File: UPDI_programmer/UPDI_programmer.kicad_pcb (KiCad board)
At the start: 2 copper layers, 74.3 x 25.4 mm, 30 parts, among them J1 UPDI, J2 ICSP, J3 USB_A, U1 ATmega168P-20AU, U2 FT230XS, Y1 16MHz

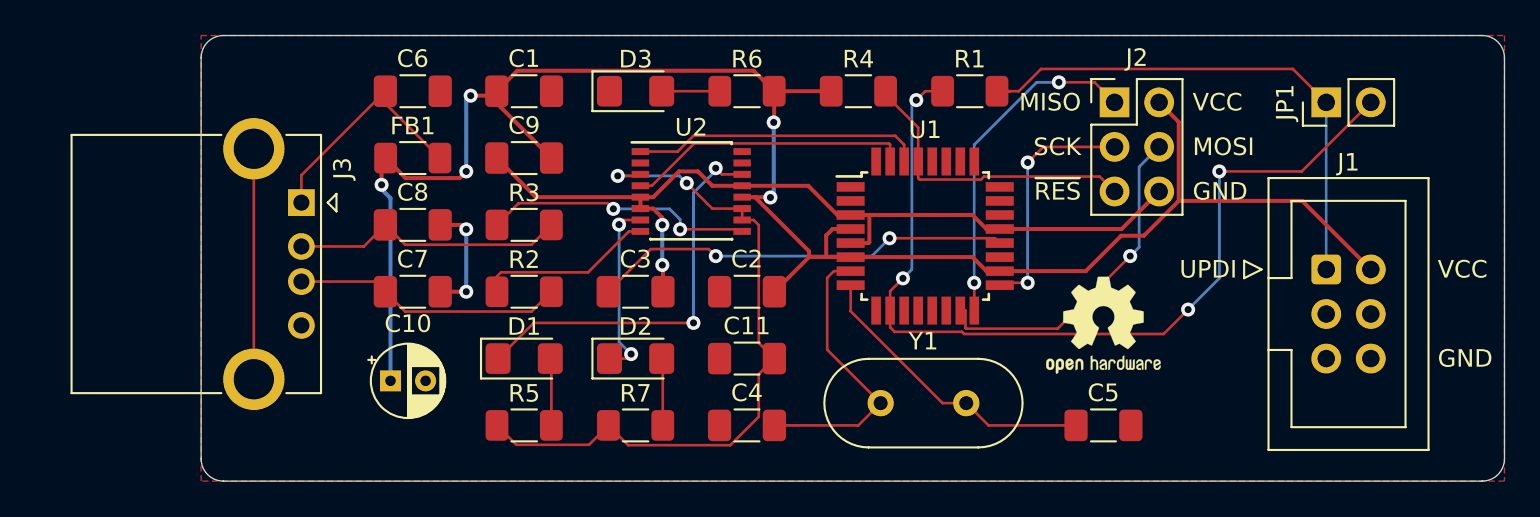
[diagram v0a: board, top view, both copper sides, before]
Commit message: UPDI PCB RC1
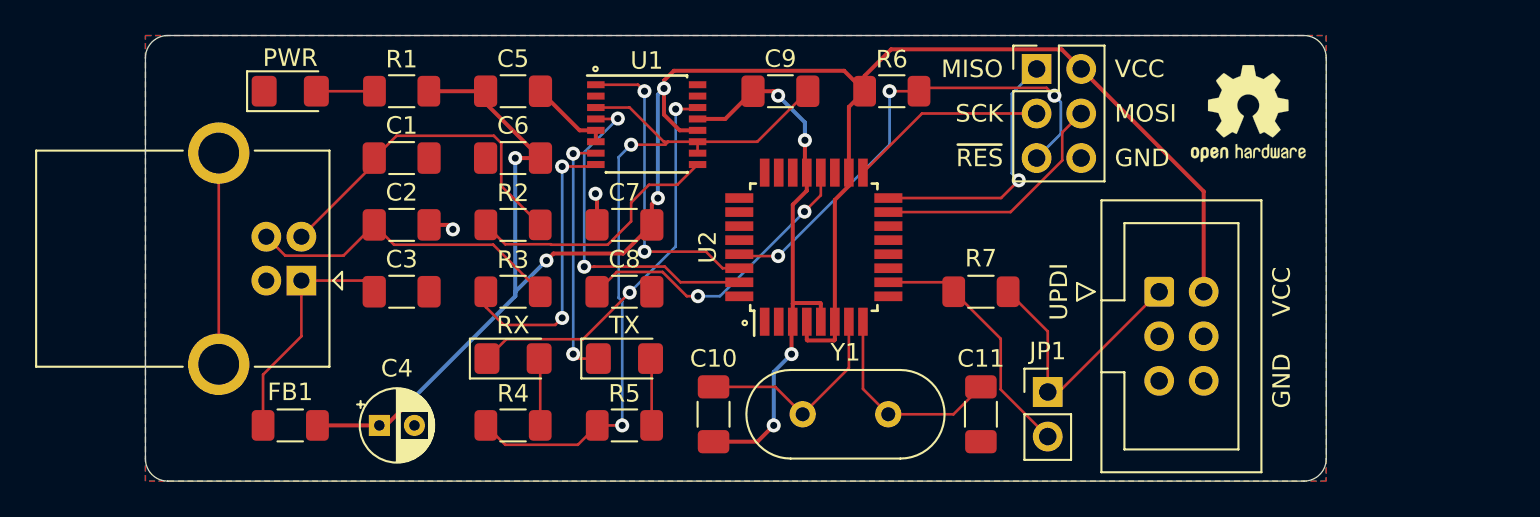
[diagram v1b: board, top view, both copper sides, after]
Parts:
- added QR*****: https://tinyurl.com/ghdbks, QR:kicad-simple, B.Cu at (160.0, 61.6)
- added REF**: KiCad-Logo2_5mm_SilkScreen, Symbol:KiCad-Logo2_5mm_SilkScreen, B.Cu at (128.9, 66.0)
- J3: value USB_A -> USB_B; footprint Connector_USB:USB_A_CONNFLY_DS1095-WNR0 -> Connector_USB:USB_B_OST_USB-B1HSxx_Horizontal
- moved JP1 22.9 mm to (150.5, 75.6), turned to 0 degrees
- moved D3 19.7 mm to (107.3, 58.4)
- moved R1 19.7 mm to (113.7, 58.4)
- moved FB1 16.8 mm to (107.3, 77.5), turned to 180 degrees
- moved C9 15.4 mm to (135.3, 58.4)
- moved REF** 14.6 mm to (161.9, 59.7)
- moved C3 11.4 mm to (113.7, 69.8)
- moved R7 11.4 mm to (146.7, 69.8)
- moved J1 9.61 mm to (156.8, 69.8)
- moved C7 7.96 mm to (126.4, 66.0)
- moved C11 7.01 mm to (146.7, 76.8), turned to 270 degrees
- moved U2 6.38 mm to (137.2, 67.3), turned to 90 degrees
- moved J2 4.84 mm to (149.9, 57.1)
- moved U1 4.58 mm to (127.6, 60.3)
- moved Y1 4.49 mm to (136.5, 76.8)
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- renumbered C8 to C1, C4 to C10, C5 to C11, C7 to C2, C6 to C3, C10 to C4, C1 to C5, C9 to C6, C2 to C7, C3 to C8, C11 to C9, R6 to R1, R3 to R2, R2 to R3, R5 to R4, R7 to R5, R4 to R6, R1 to R7, U2 to U1, U1 to U2
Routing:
- net UPDI: track 51.9 -> 14.4 mm, vias 4 -> 0
- net GND: track 58.2 -> 40.1 mm, vias 4 -> 6
- net Net-(J1-Pad1): track 30.3 -> 15.4 mm
- net ~RESET: track 17.4 -> 28.2 mm, vias 0 -> 3
- net Net-(C8-Pad1): track 24.0 -> 17.5 mm
- net USBD+: track 10.1 -> 16.4 mm, vias 0 -> 2
- net Net-(C11-Pad1): track 17.0 -> 11.8 mm
- net MOSI: track 19.3 -> 14.3 mm, vias 1 -> 0
- net MISO: track 19.4 -> 15.0 mm, vias 2 -> 1
- net Net-(C10-Pad2): track 16.5 -> 12.1 mm
- net VCC: track 109.1 -> 113.5 mm
- net Net-(C1-Pad1): track 15.7 -> 19.7 mm
- net ~TXLED: track 10.3 -> 14.3 mm
- net TxD: track 16.2 -> 19.7 mm, vias 0 -> 2
- net Net-(C2-Pad1): track 15.4 -> 18.4 mm
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- added copper zone on B.Cu, net GND
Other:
- board size 74.3 x 25.4 mm -> 67.3 x 25.4 mm
- board text added: "Based on Stefan Wagner’s design https://easyeda.com/wagiminator/y-updi-programmer"
- board text added: "JTAG2UPDI Programmer ver. 1.0 Designed by Dawid Buchwald"
- board text added: "PWR"
- board text added: "RX"
- board text added: "TX"
